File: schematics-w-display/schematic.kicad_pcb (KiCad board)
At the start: 2 copper layers, 61 x 63.1 mm, 8 parts, among them J1 Conn_01x21_Female, J2 Conn_01x06_Female, J3 Conn_01x21_Female, J4 Conn_01x08_Female

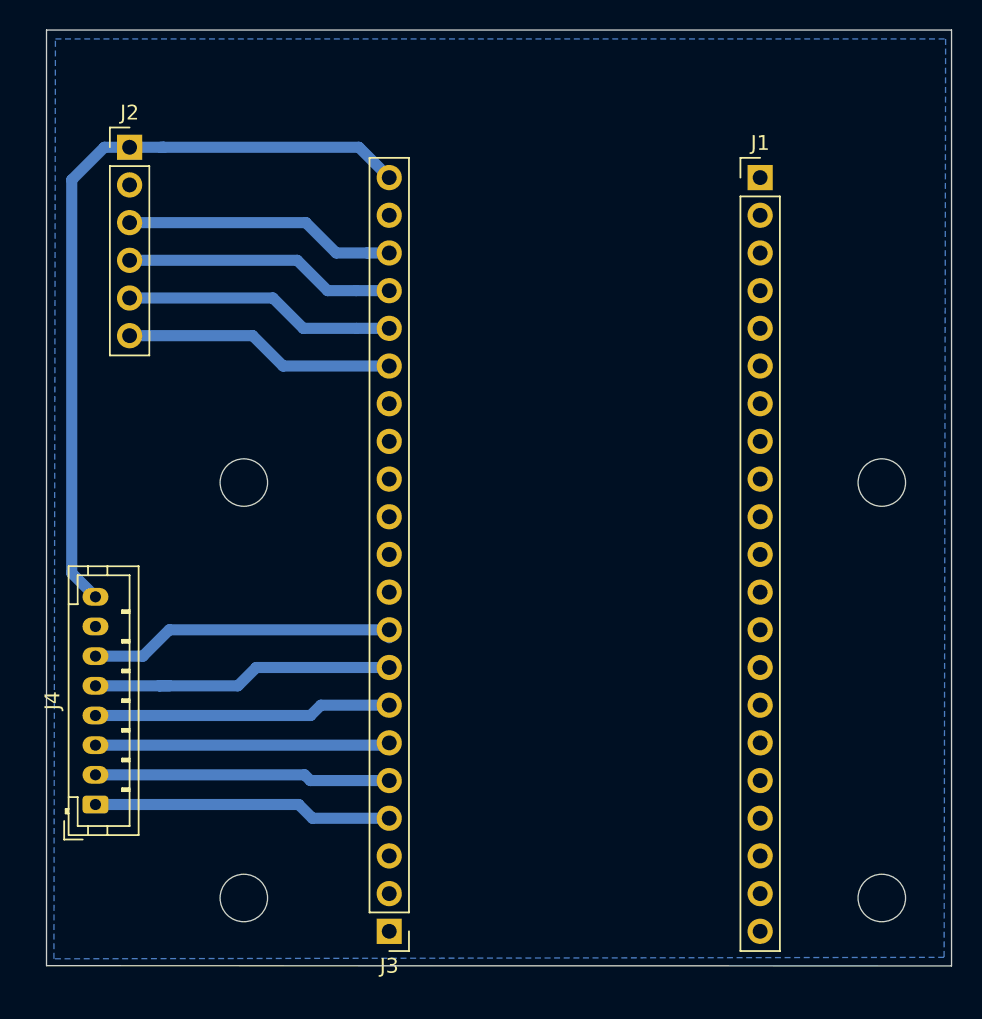
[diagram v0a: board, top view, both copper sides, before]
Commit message: v4
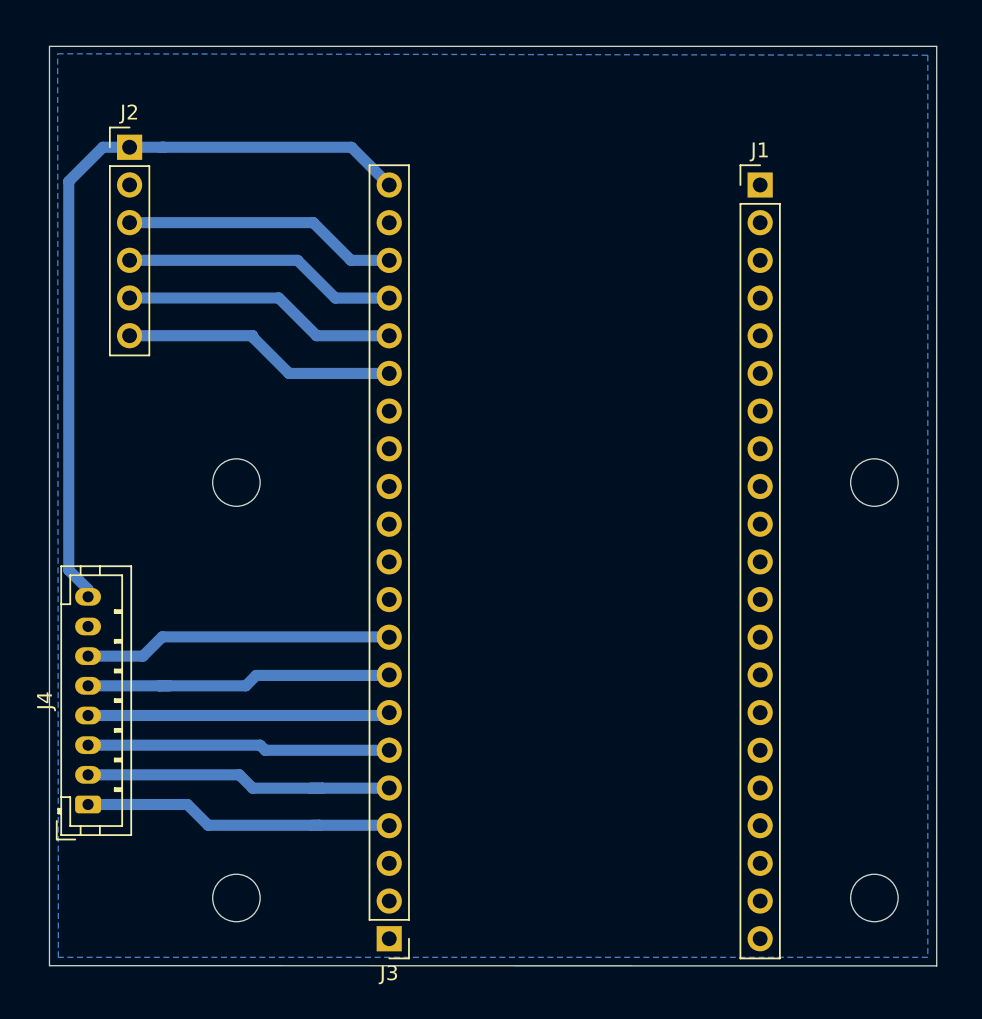
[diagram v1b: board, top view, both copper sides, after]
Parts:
- moved   0.50 mm to (99.7, 90.5)
- moved   0.50 mm to (99.7, 118.5)
- moved   0.50 mm to (142.7, 118.5)
- moved   0.50 mm to (142.7, 90.5)
- moved J1 0.50 mm to (135.0, 70.4)
- moved J3 0.50 mm to (110.0, 121.2)
- moved J4 0.50 mm to (89.7, 112.2)
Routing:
- net /RST: track 20.0 -> 21.0 mm
- net /BUSY: track 20.2 -> 20.9 mm
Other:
- board size 61 x 63.1 mm -> 59.8 x 62 mm

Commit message: Final version
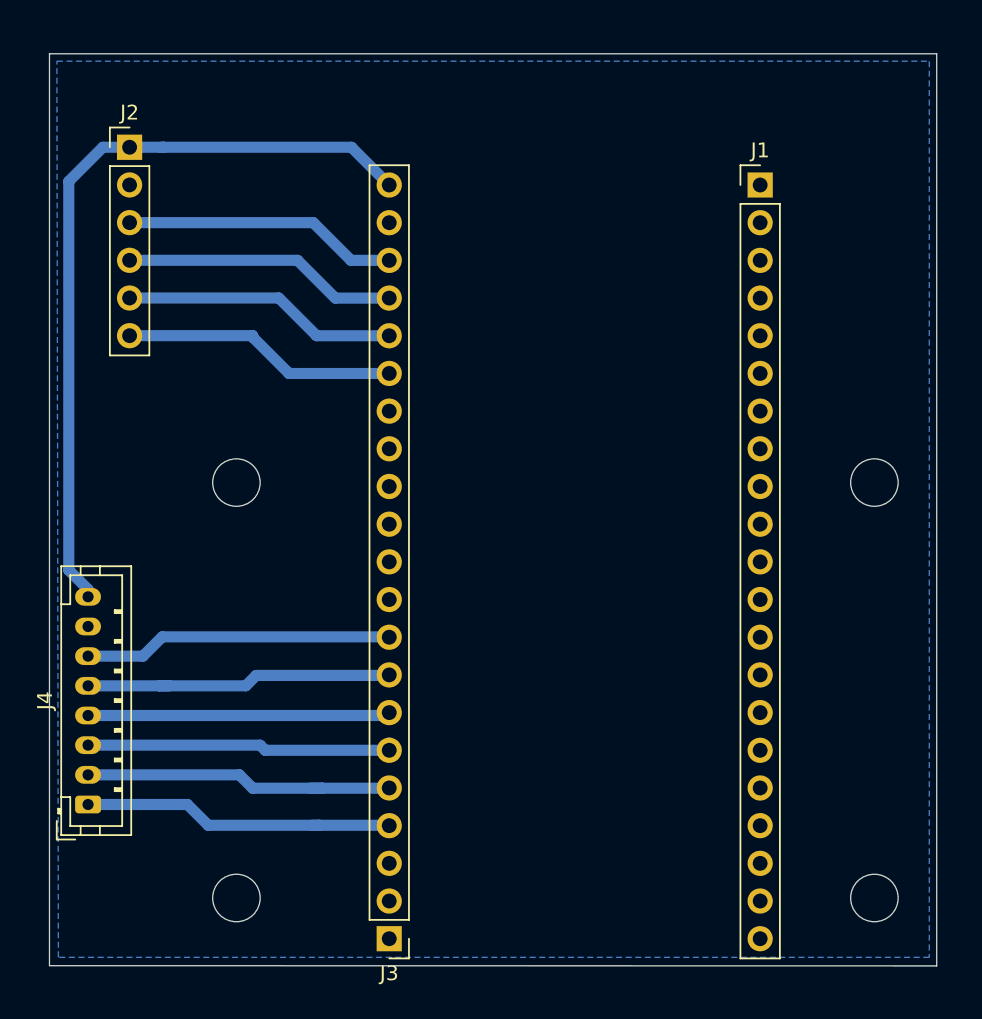
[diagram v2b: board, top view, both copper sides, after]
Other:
- board size 59.8 x 62 mm -> 59.8 x 61.5 mm
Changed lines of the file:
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@@
   )
   (gr_line (start 87.1 123.063) (end 146.9 123.079) (layer Edge.Cuts) (width 0.05))
-  (gr_line (start 146.9 61.1) (end 87.1 61.1) (layer Edge.Cuts) (width 0.05))
-  (gr_line (start 87.1 61.1) (end 87.1 123.063) (layer Edge.Cuts) (width 0.05))
-  (gr_line (start 146.9 123.079) (end 146.9 61.1) (layer Edge.Cuts) (width 0.05))
+  (gr_line (start 146.9 61.6) (end 87.1 61.6) (layer Edge.Cuts) (width 0.05))
+  (gr_line (start 87.1 61.6) (end 87.1 123.063) (layer Edge.Cuts) (width 0.05))
+  (gr_line (start 146.9 123.079) (end 146.9 61.6) (layer Edge.Cuts) (width 0.05))
   (segment (start 92.5 67.9) (end 94.8 67.9) (width 0.75) (layer B.Cu) (net 1))
   (segment (start 94.8 67.9) (end 94.6 67.9) (width 0.75) (layer B.Cu) (net 1))
@@
     (polygon
       (pts
-        (xy 146.3 122.5) (xy 87.7 122.5) (xy 87.65 61.6) (xy 146.3 61.7)
+        (xy 146.4 122.5) (xy 87.7 122.5) (xy 87.6 62.1) (xy 146.4 62.1)
       )
     )
